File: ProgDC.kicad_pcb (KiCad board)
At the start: 2 copper layers, 145 x 100 mm, 45 parts, among them J1 Conn_02x20_Counter_Clockwise_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, J2 Conn_01x24_Pin, J3 Conn_01x03_Pin, U1 KR580VK28, U2 628512, U3 CPU

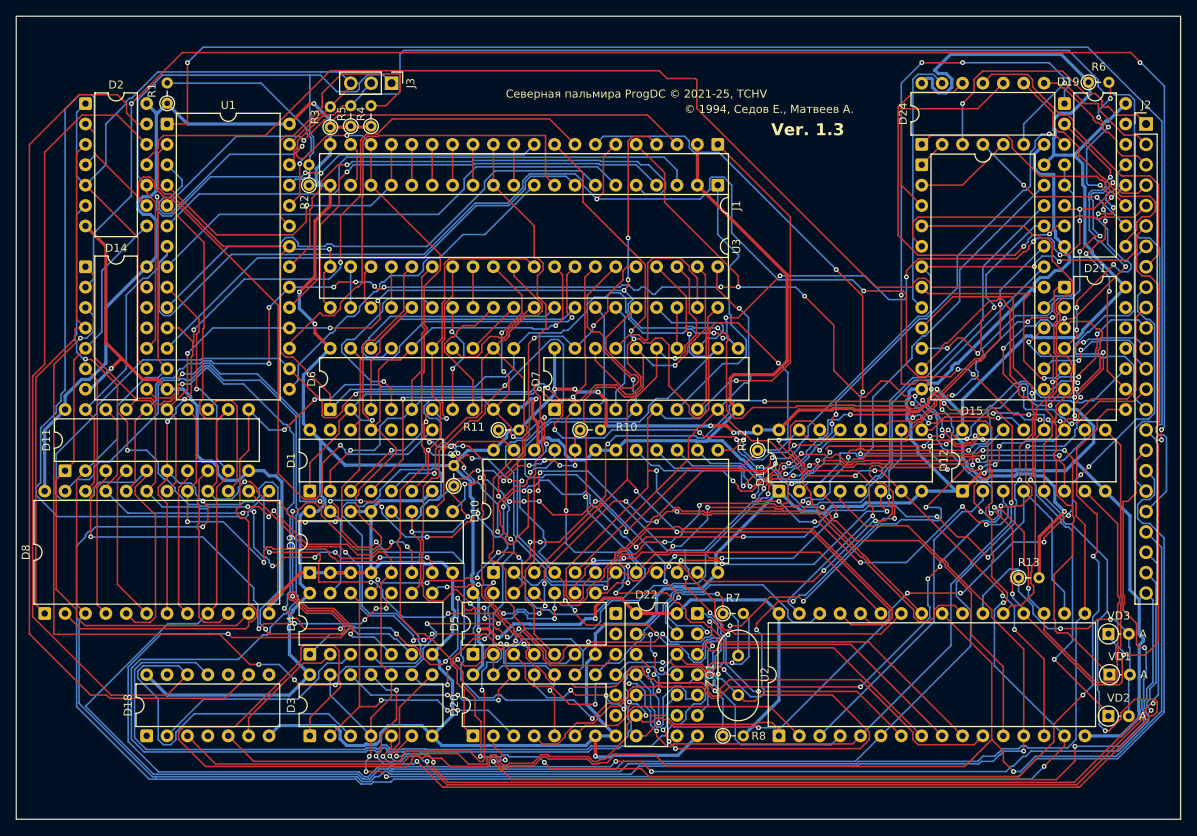
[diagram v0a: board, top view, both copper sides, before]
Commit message: Ver. 1.4
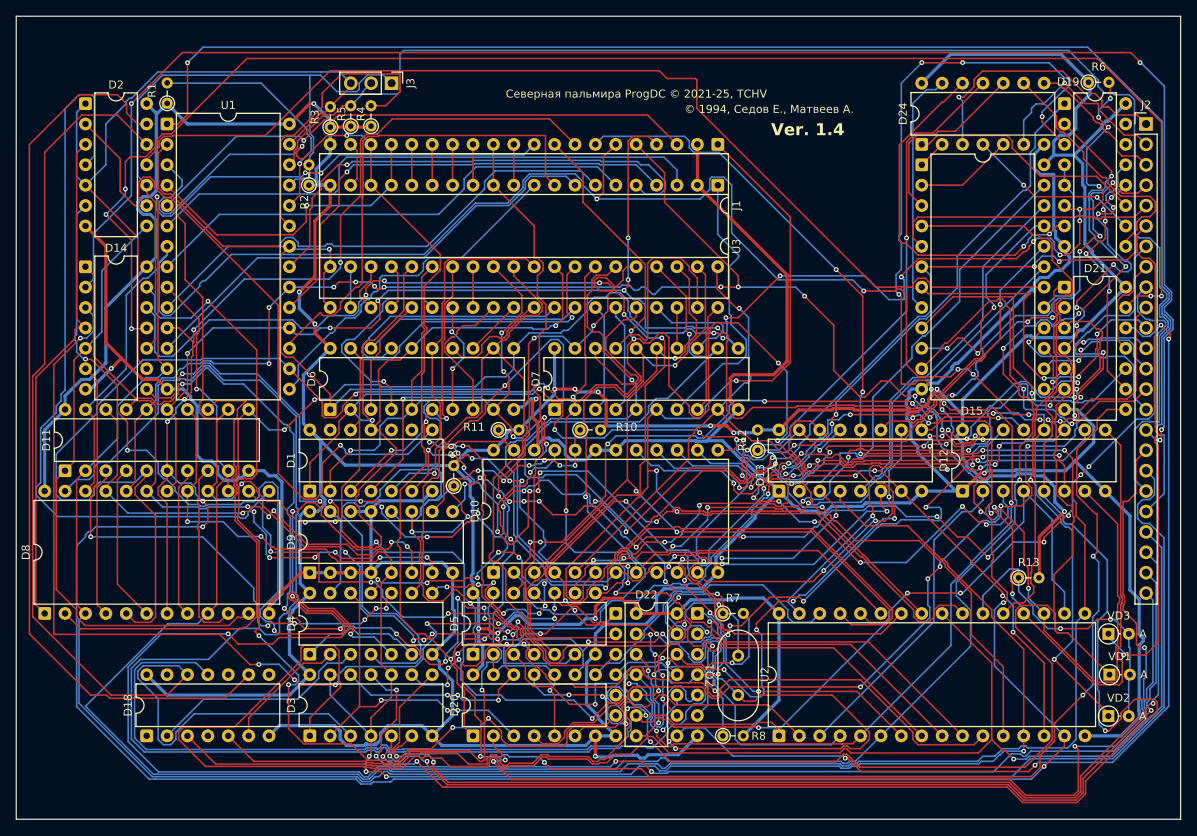
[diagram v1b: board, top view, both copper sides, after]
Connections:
- D14 pad 11: unconnected-(D14.4-Y-Pad11) -> Net-(D14.4-Y)
- D14 pad 12: unconnected-(D14.4-A-Pad12) -> Net-(D14.4-A)
- D14 pad 13: unconnected-(D14.4-B-Pad13) -> Net-(D14.4-B)
- D19 pad 1: /AB7 -> /AB5
- D19 pad 3: /AB5 -> /AB7
- D21 pad 11: unconnected-(D21.4-Y-Pad11) -> /~{CS_DMA_2}
- D21 pad 12: unconnected-(D21.4-A-Pad12) -> Net-(D21.4-A)
- D21 pad 13: unconnected-(D21.4-B-Pad13) -> Net-(D14.4-Y)
- D22 pad 1: unconnected-(D22.1-A-Pad1) -> /~{WR}
- D22 pad 2: unconnected-(D22.1-Y-Pad2) -> Net-(D14.4-A)
- D22 pad 5: unconnected-(D22.3-A-Pad5) -> /~{CS_RAMR}
- D22 pad 6: unconnected-(D22.3-Y-Pad6) -> Net-(D14.4-B)
- D22 pad 8: unconnected-(D22.4-Y-Pad8) -> Net-(D21.4-A)
- D22 pad 9: unconnected-(D22.4-A-Pad9) -> /~{CS_DMA_}
- J2 pad 8: /~{CS_DMA_} -> /~{CS_DMA_2}
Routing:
- net Net-(D14.4-Y): track 0.00 -> 189.8 mm, vias 0 -> 5
- net Net-(D14.4-A): track 0.00 -> 135.9 mm, vias 0 -> 5
- net Net-(D14.4-B): track 0.00 -> 122.8 mm, vias 0 -> 5
- net Net-(D21.4-A): track 0.00 -> 120.7 mm, vias 0 -> 4
- net /~{CS_RAMR}: track 82.3 -> 170.5 mm, vias 0 -> 1
- net /~{CS_DMA_}: track 40.0 -> 107.5 mm, vias 0 -> 8
- net /~{WR}: track 127.3 -> 152.2 mm, vias 2 -> 6
- net /~{CS_DMA_2}: track 0.00 -> 12.5 mm
- net /AB7: track 283.9 -> 291.7 mm, vias 11 -> 12
- net +5V: track 525.0 -> 518.8 mm
- net /AB15: track 52.7 -> 58.4 mm
- net /AB4: track 140.2 -> 145.4 mm
- net /AB5: track 213.7 -> 218.1 mm, vias 15 -> 14
- net /8MHZ: track 110.0 -> 114.1 mm
- net /~{MEMW_VT57}: track 128.6 -> 132.6 mm
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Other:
- board text added: "Ver. 1.4"
- board text removed: "Ver. 1.3"

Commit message: Fix
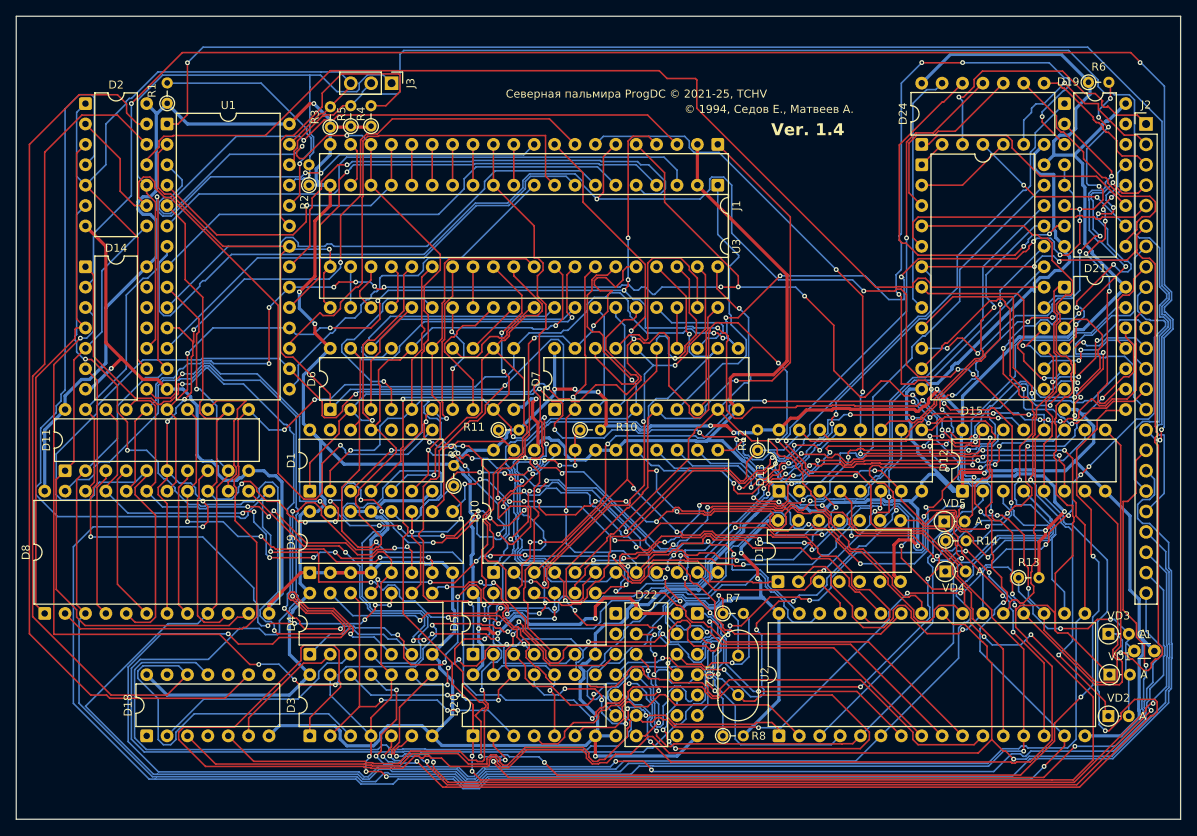
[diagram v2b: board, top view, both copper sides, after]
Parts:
- added C1: 470, Capacitor_THT:C_Disc_D3.0mm_W1.6mm_P2.50mm, F.Cu at (181.4, 111.4)
- added D16: 133LL1, Package_DIP:DIP-14_W7.62mm, F.Cu at (137.0, 102.7)
- added R14: R0125, Resistor_THT:R_Axial_DIN0204_L3.6mm_D1.6mm_P2.54mm_Vertical, F.Cu at (157.9, 97.6)
- added VD4: 1N4148, Diode_THT:D_DO-34_SOD68_P2.54mm_Vertical_AnodeUp, F.Cu at (157.9, 101.4)
- added VD5: 1N4148, Diode_THT:D_DO-34_SOD68_P2.54mm_Vertical_AnodeUp, F.Cu at (157.8, 95.2)
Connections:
- D14 pad 11: Net-(D14.4-Y) -> unconnected-(D14.4-Y-Pad11)
- D14 pad 12: Net-(D14.4-A) -> unconnected-(D14.4-A-Pad12)
- D14 pad 13: Net-(D14.4-B) -> unconnected-(D14.4-B-Pad13)
- D21 pad 12: Net-(D21.4-A) -> GND
- D21 pad 13: Net-(D14.4-Y) -> Net-(D21.4-B)
- D22 pad 1: /~{WR} -> unconnected-(D22.1-A-Pad1)
- D22 pad 2: Net-(D14.4-A) -> unconnected-(D22.1-Y-Pad2)
- D22 pad 6: Net-(D14.4-B) -> /CS_RAMR
- D22 pad 8: Net-(D21.4-A) -> unconnected-(D22.4-Y-Pad8)
- D22 pad 9: /~{CS_DMA_} -> unconnected-(D22.4-A-Pad9)
- D4 pad 13: Net-(D14.3-Y) -> Net-(D16.4-Y)
- U2 pad 29: /~{WE_628512} -> Net-(D16.1-Y)
- U2 pad 31: /R3 -> /AB15
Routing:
- net Net-(D14.4-Y): track 189.8 -> 0.00 mm, vias 5 -> 0
- net Net-(D14.4-A): track 135.9 -> 0.00 mm, vias 5 -> 0
- net Net-(D14.4-B): track 122.8 -> 0.00 mm, vias 5 -> 0
- net Net-(D21.4-A): track 120.7 -> 0.00 mm, vias 4 -> 0
- net /~{WR}: track 152.2 -> 265.5 mm, vias 6 -> 7
- net Net-(D16.4-Y): track 0.00 -> 73.7 mm, vias 0 -> 4
- net Net-(D14.3-Y): track 51.3 -> 106.0 mm, vias 2 -> 9
- net /CS_RAMR: track 0.00 -> 53.6 mm
- net Net-(D21.4-B): track 0.00 -> 50.0 mm, vias 0 -> 1
- net /AB15: track 58.4 -> 104.7 mm, vias 3 -> 8
- net /R3: track 83.6 -> 42.8 mm, vias 2 -> 1
- net GND: track 510.5 -> 546.9 mm, vias 4 -> 6
- net /~{CS_628512}: track 38.7 -> 75.1 mm, vias 2 -> 3
- net /~{WE_628512}: track 89.9 -> 59.3 mm
- net /~{CS_RAMR}: track 170.5 -> 197.9 mm, vias 1 -> 6
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
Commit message: Fix layout
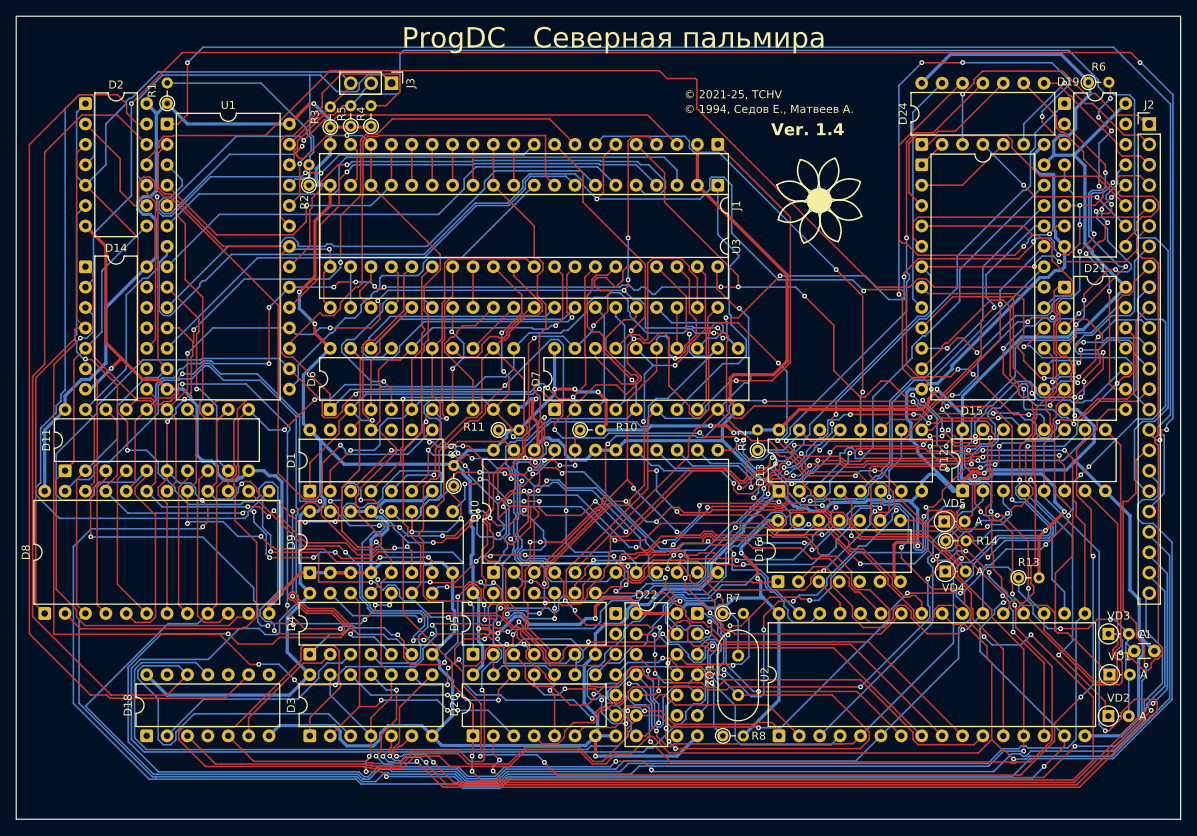
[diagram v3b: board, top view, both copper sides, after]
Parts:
- moved J2 0.40 mm to (183.3, 45.7)
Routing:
- net /DB4: track 290.5 -> 282.4 mm
- net Net-(D19-3): track 35.7 -> 31.4 mm
- net GND: track 546.9 -> 542.8 mm
- net /AB7: track 301.5 -> 297.9 mm
- net Net-(D14.1-A): track 122.0 -> 119.0 mm
- net /AB10: track 142.5 -> 139.7 mm
- net /"1": track 216.7 -> 214.0 mm
- net /C800_VI53_2: track 150.0 -> 147.5 mm
- net /CLK: track 170.6 -> 168.2 mm
- net /~{RD}: track 216.9 -> 214.7 mm
- net Net-(D21.2-A): track 35.3 -> 33.2 mm
- net Net-(D22.5-Y): track 65.7 -> 63.9 mm
- net /8MHZ: track 111.7 -> 109.9 mm
- net Net-(D20.2-A): track 116.7 -> 114.9 mm
- net Net-(D21.1-B): track 105.9 -> 104.3 mm
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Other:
- board text added: "ProgDC Северная пальмира"
- board text added: "© 2021-25, TCHV"
- board text removed: "Северная пальмира ProgDC © 2021-25, TCHV"
